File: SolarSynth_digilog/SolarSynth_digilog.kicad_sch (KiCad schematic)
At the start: 31 parts, among them J1 OutputJack1, J2 Conn_01x01_Pin, J3 Conn_01x01_Pin, P1 PiezoDisc, P2 PiezoDisc, U1 74HC14, U2 MCP6002-xMC

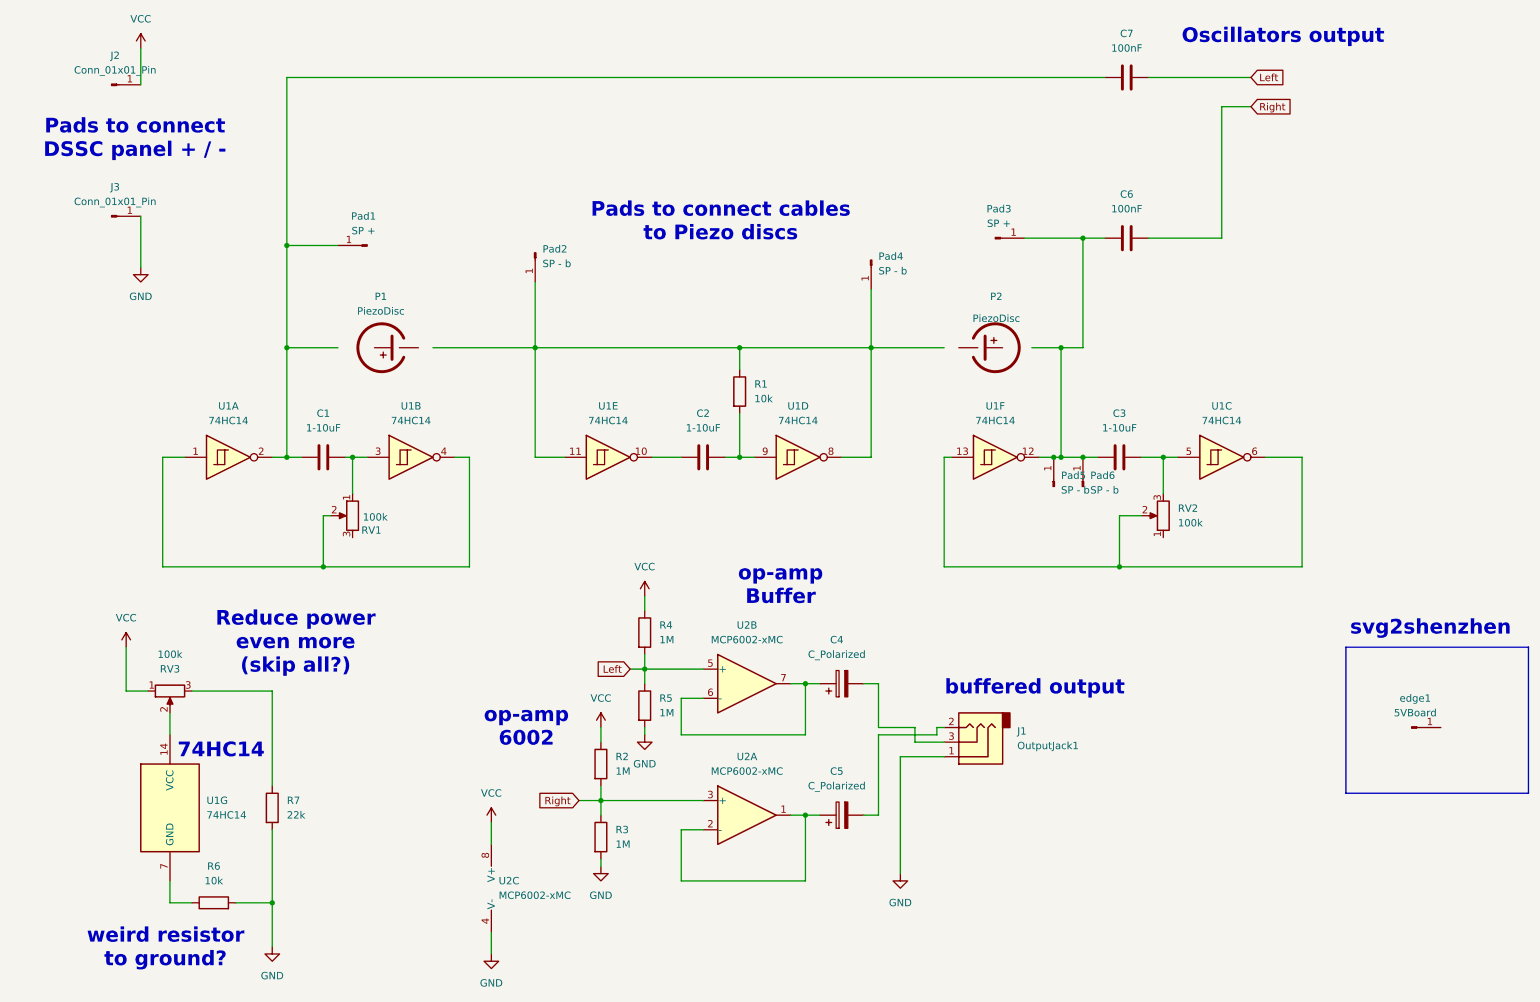
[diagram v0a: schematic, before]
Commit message: added original digilog again and moved THT-Version to a new folder
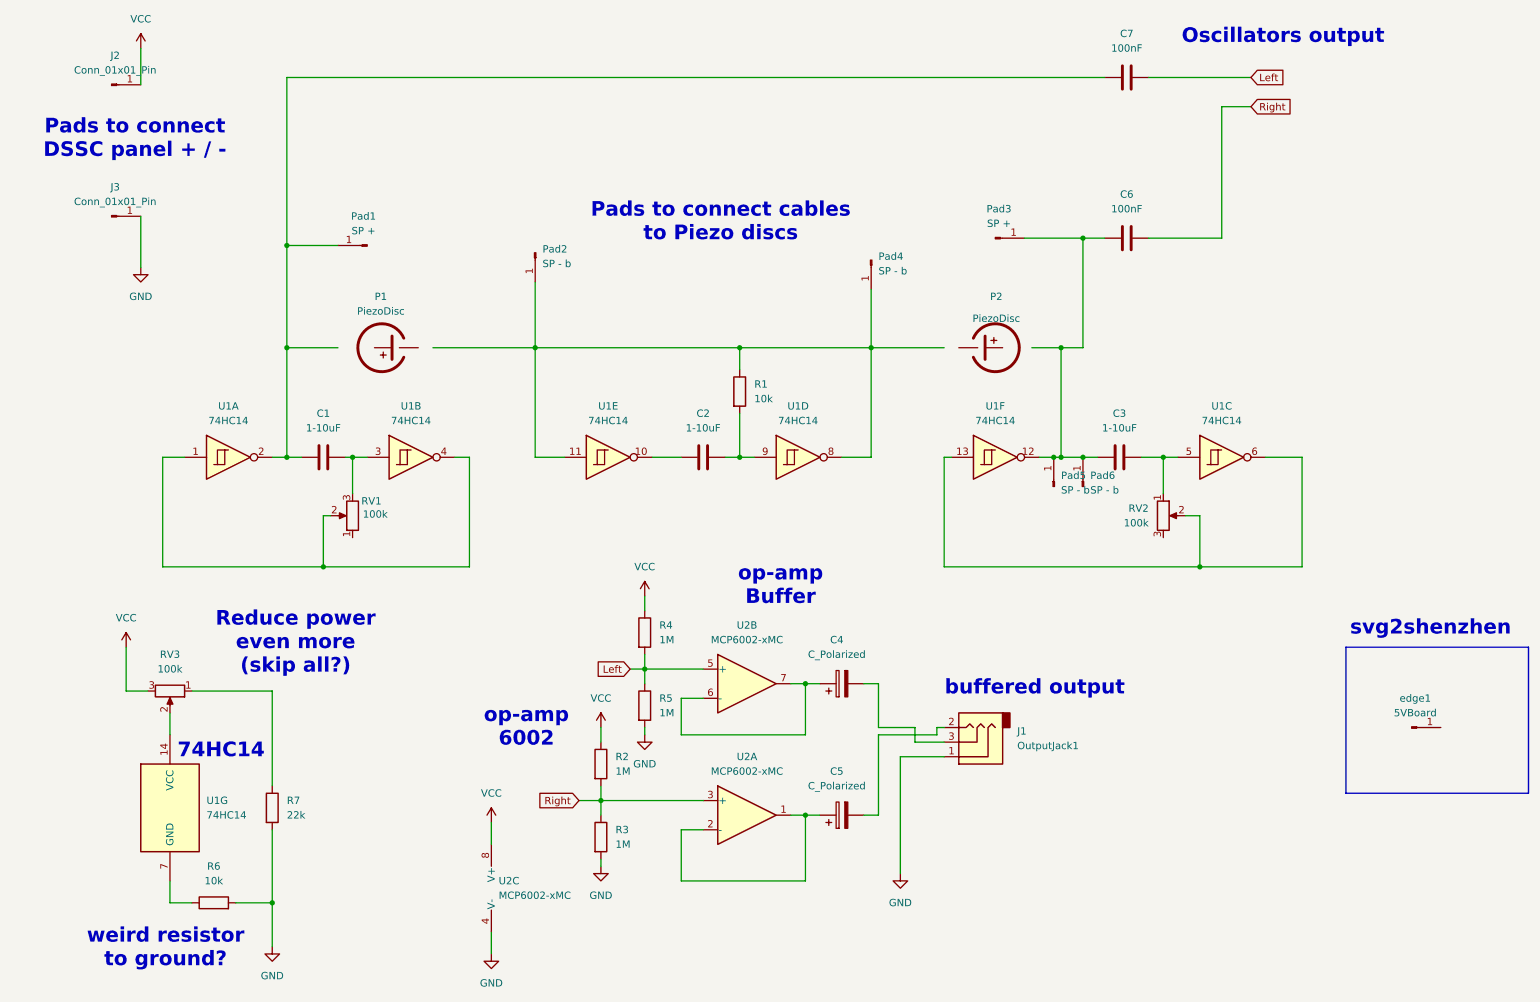
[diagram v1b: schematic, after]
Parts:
- C1, C2, C3: footprint Capacitor_THT:C_Disc_D5.0mm_W2.5mm_P5.00mm -> 007_dusjagr:C_1210_noGND
- C4, C5: footprint Capacitor_THT:CP_Radial_D5.0mm_P2.50mm -> 007_dusjagr:C_1210_noGND
- C6, C7: footprint Capacitor_THT:C_Disc_D5.0mm_W2.5mm_P2.50mm -> 007_dusjagr:C_1210_noGND
- J1: footprint 002_Solarpunk:AUDIO-JACK-3.5mm_SMD_noHole -> 007_dusjagr:AUDIO-JACK-3.5mm_SMD_noHole
- J2, J3: footprint 002_Solarpunk:SolarPad_VCC -> 007_dusjagr:SolarPad_VCC
- Pad1, Pad2, Pad3, Pad4, Pad5, Pad6: footprint 002_Solarpunk:SolderPad_small -> 007_dusjagr:SolderPad_small
- R1, R2, R3, R4, R5, R6, R7: footprint Resistor_THT:R_Axial_DIN0309_L9.0mm_D3.2mm_P12.70mm_Horizontal -> 007_dusjagr:R_1206_noGND
- RV1, RV2: footprint blinkyparts:Potentiometer_Alpha_RD901F-40-00D_Single_Vertical_bigger-holes -> 007_dusjagr:RD901F-ALPHA-3D_minis
- RV3: footprint blinkyparts:Potentiometer_Alpha_RD901F-40-00D_Single_Vertical_bigger-holes -> 007_dusjagr:RD901F-ALPHA-3D_longpads
- U1: footprint 002_Solarpunk:DIP-14_W7.62mm_LongerPads -> 007_dusjagr:DIP-14_W7.62mm_LongerPads
- U2: footprint Package_DIP:DIP-8_W7.62mm_LongPads -> 007_dusjagr:DIP-8_W7.62mm_LongerPads
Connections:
- net VCC: now also RV3.3; no longer RV3.1
- net at C1.2, U1.3: now also RV1.3; no longer RV1.1
- net at C3.2, U1.5: now also RV2.1; no longer RV2.3
- net at R7.1: now also RV3.1; no longer RV3.3
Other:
- moved on the sheet: RV1, RV2, RV3
